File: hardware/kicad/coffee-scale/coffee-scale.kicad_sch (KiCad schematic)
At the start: 7 parts, among them J1 Screw_Terminal_01x02, U1 ESP32-S3, U2 HX711, U4 MCP73831-2-MC

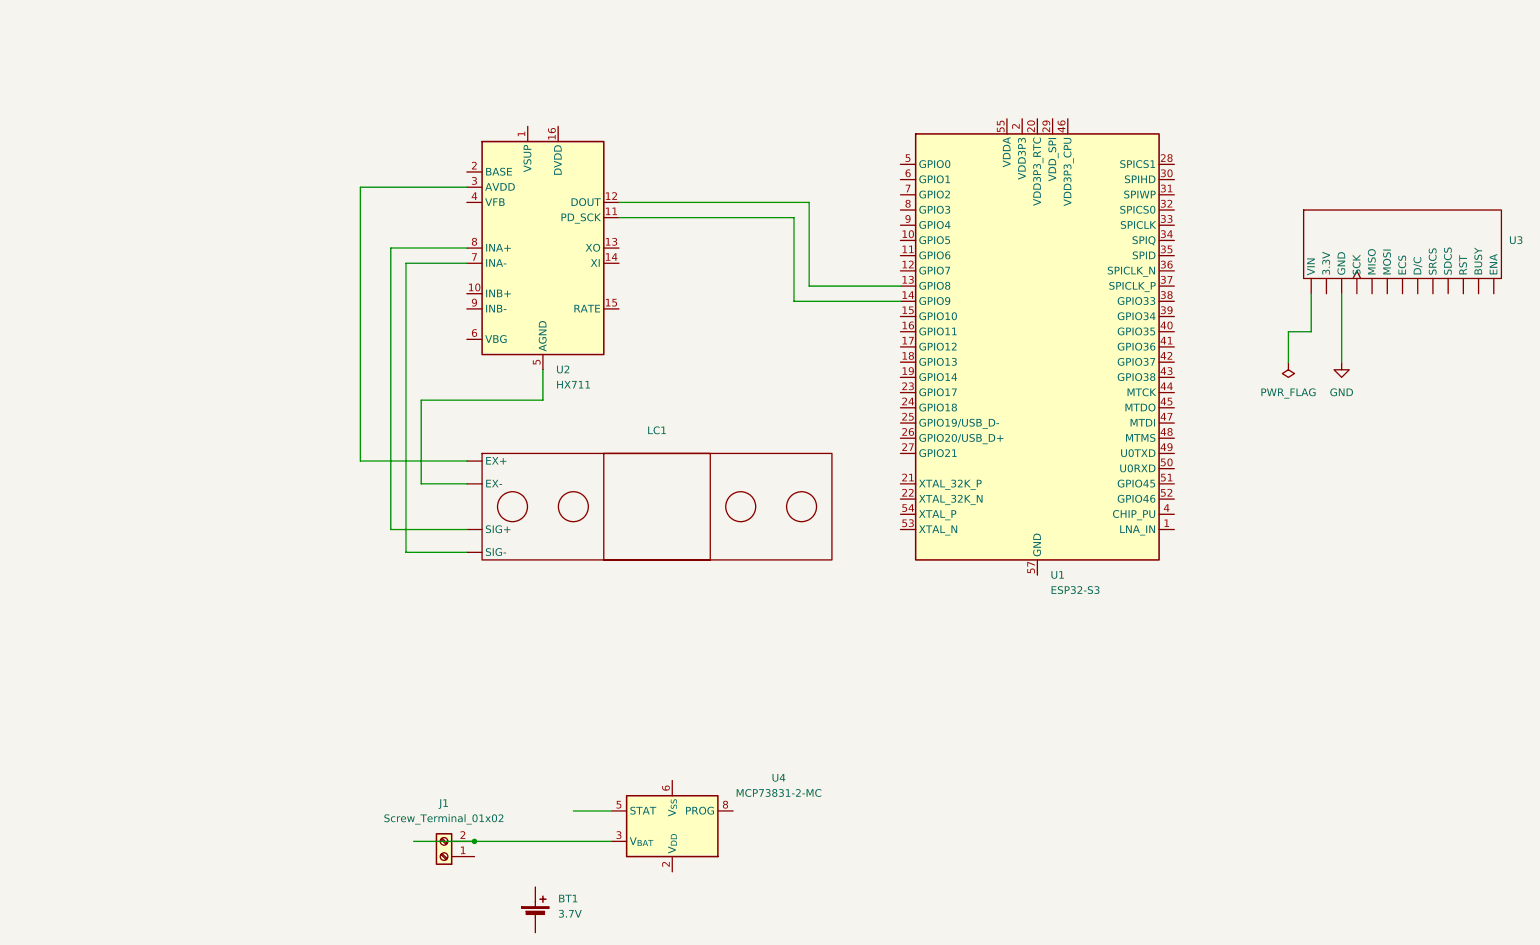
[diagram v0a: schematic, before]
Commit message: Update on KiCad
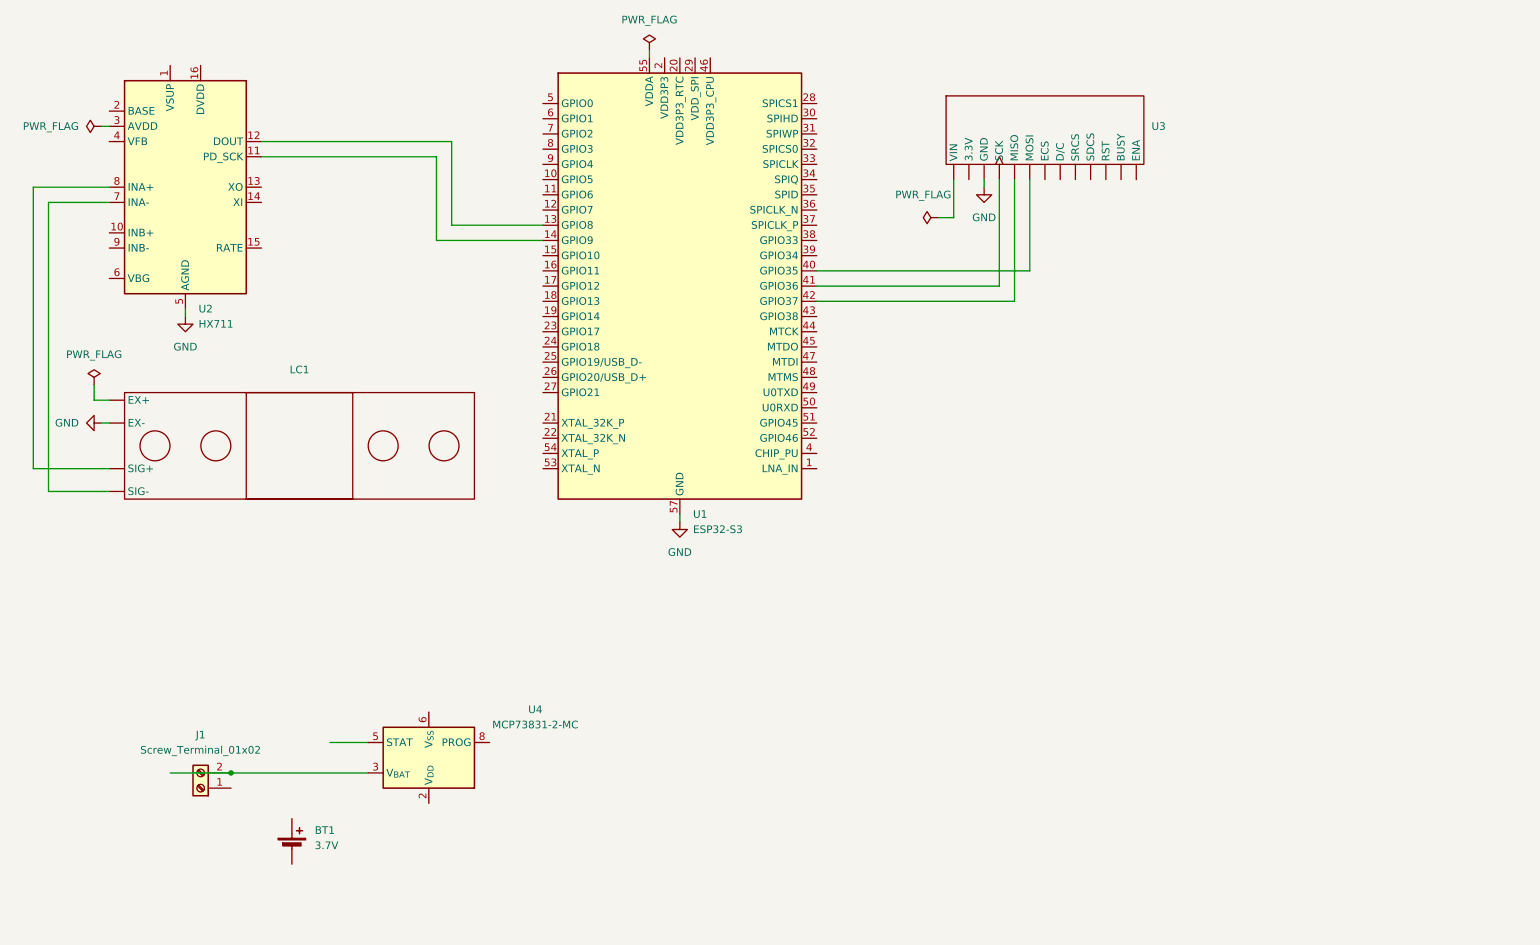
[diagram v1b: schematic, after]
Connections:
- net GND: now also LC1. (SIG-), U1.57 (GND), U2.5 (AGND)
- net at U1.40 (GPIO35): now also U3. (VIN)
- net at U1.41 (GPIO36): now also U3. (VIN)
- net at U1.42 (GPIO37): now also U3. (VIN)
- net at U2.3 (AVDD): no longer LC1. (SIG-)
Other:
- moved on the sheet: BT1, J1, LC1, U1, U2, U3, U4
